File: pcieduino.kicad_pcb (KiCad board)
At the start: 2 copper layers, 51 x 30 mm, 29 parts, among them J1 PCIE-MINI, J2 ISP, J3 DIGITAL, J4 ANALOG_POWER, SW1 SW_PUSH, U1 ATMEGA32U4-AU, X1 8MHz

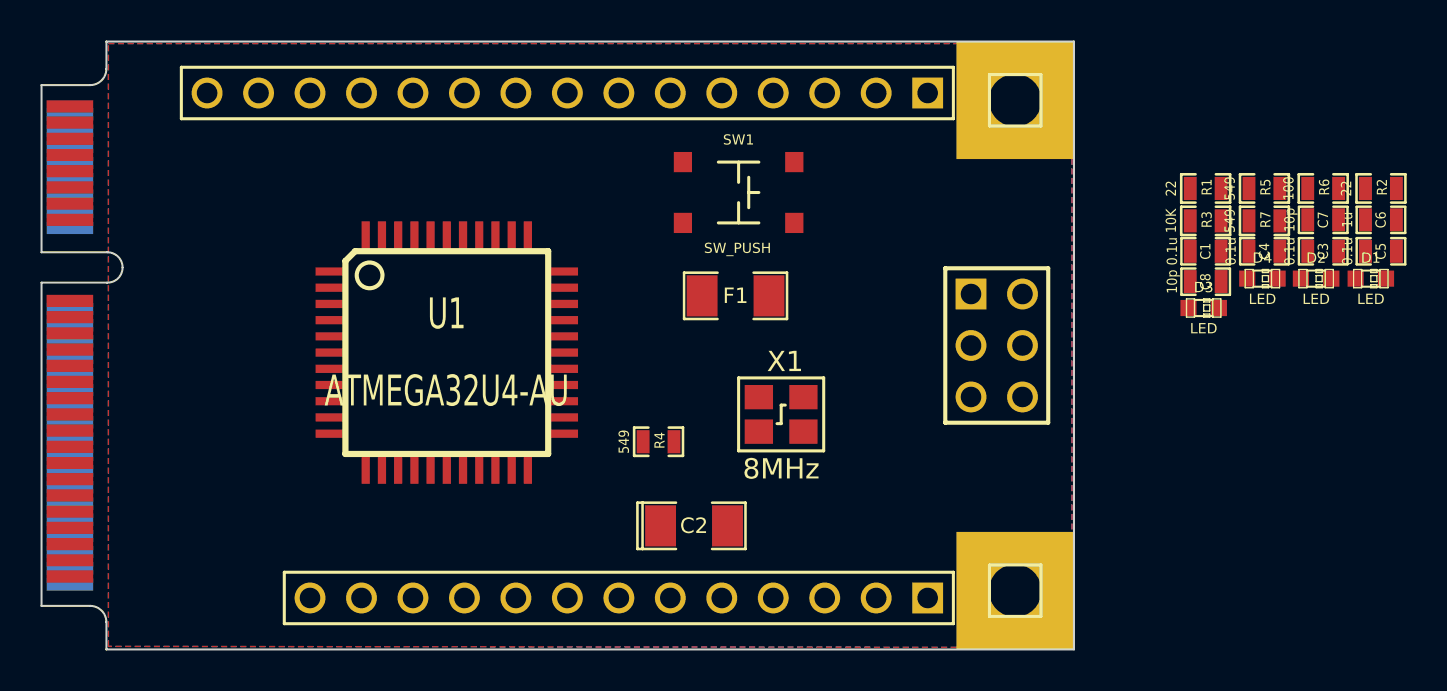
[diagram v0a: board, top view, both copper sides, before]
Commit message: work in progress, after autorouting and all connections
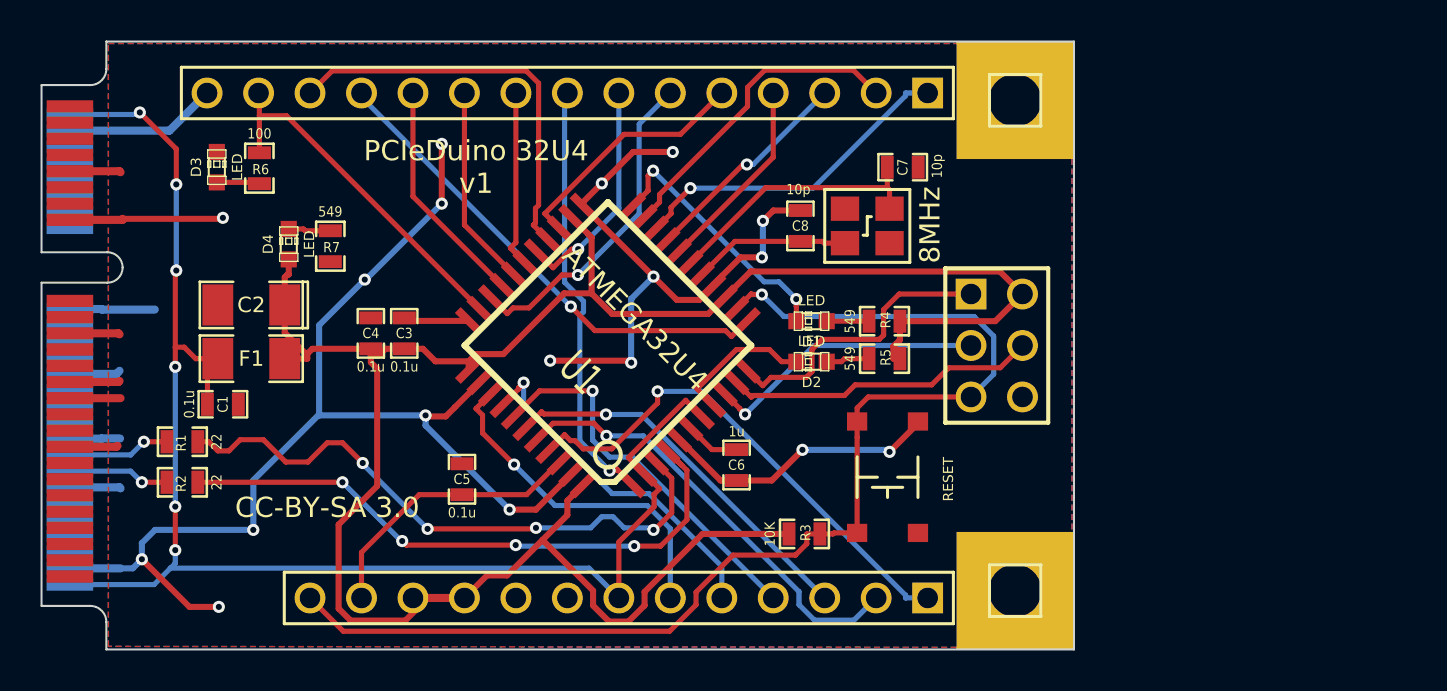
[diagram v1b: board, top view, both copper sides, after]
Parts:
- SW1: value SW_PUSH -> RESET
- U1: value ATMEGA32U4-AU -> ATMEGA32U4
- moved R2 60.9 mm to (56.0, 121.8), turned to 180 degrees
- moved R6 52.5 mm to (59.8, 106.2), turned to 270 degrees
- moved R1 52.0 mm to (56.0, 119.8), turned to 180 degrees
- moved D3 49.2 mm to (57.7, 106.2), turned to 90 degrees
- moved C1 49.1 mm to (58.0, 117.9)
- moved D4 48.1 mm to (61.2, 110.0), turned to 90 degrees
- moved C5 46.7 mm to (69.8, 121.6), turned to 90 degrees
- moved R7 46.1 mm to (63.3, 110.1), turned to 270 degrees
- moved C3 45.5 mm to (67.0, 114.4), turned to 90 degrees
- moved C4 44.3 mm to (65.3, 114.4), turned to 90 degrees
- moved C6 34.0 mm to (83.3, 120.9), turned to 270 degrees
- moved D1 27.7 mm to (87.0, 113.8), turned to 180 degrees
- moved D2 25.2 mm to (87.0, 115.8), turned to 180 degrees
- moved R3 25.1 mm to (86.7, 124.3)
- moved C2 24.4 mm to (59.4, 113.0), turned to 180 degrees
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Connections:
- J1 pad 36: N-000003 -> N-000002
- R1 pad 1: N-000003 -> /D-
- R1 pad 2: /D- -> N-000002
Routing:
- net GND: track 0.00 -> 143.4 mm, vias 0 -> 18
- net VCC: track 0.00 -> 105.5 mm
- net /UVCC: track 0.00 -> 73.0 mm, vias 0 -> 6
- net /RESET: track 0.00 -> 59.7 mm, vias 0 -> 1
- net /D+: track 0.00 -> 30.2 mm, vias 0 -> 4
- net /D-: track 0.00 -> 30.2 mm, vias 0 -> 4
- net /A5: track 0.00 -> 25.1 mm, vias 0 -> 1
- net /D11: track 0.00 -> 24.4 mm, vias 0 -> 1
- net /A4: track 0.00 -> 21.9 mm, vias 0 -> 1
- net /D7: track 0.00 -> 21.2 mm, vias 0 -> 1
- net /D12: track 0.00 -> 20.2 mm
- net /A2: track 0.00 -> 18.9 mm, vias 0 -> 1
- net /A3: track 0.00 -> 18.9 mm, vias 0 -> 1
- net /D13: track 0.00 -> 17.8 mm
- net /A1: track 0.00 -> 17.2 mm, vias 0 -> 1
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- added copper zone on B.Cu, net GND
- removed copper zone on B.Cu, net VCC
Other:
- net class Default: via_dia 0.762 -> 0.6
- net class PCI: trace_width 0.4 -> 0.3; via_dia 0.762 -> 0.6
- net class Power: trace_width 0.4 -> 0.3; via_dia 0.889 -> 0.6; via_drill 0.635 -> 0.3048
- board text added: "CC-BY-SA 3.0"
- board text added: "PCIeDuino 32U4 v1"
